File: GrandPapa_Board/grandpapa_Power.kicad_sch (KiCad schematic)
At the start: 31 parts, among them U1 LT1576IS8-5#TRPBF, U11 INA180, U2 TPS61023DRLT, U5 FPF2124

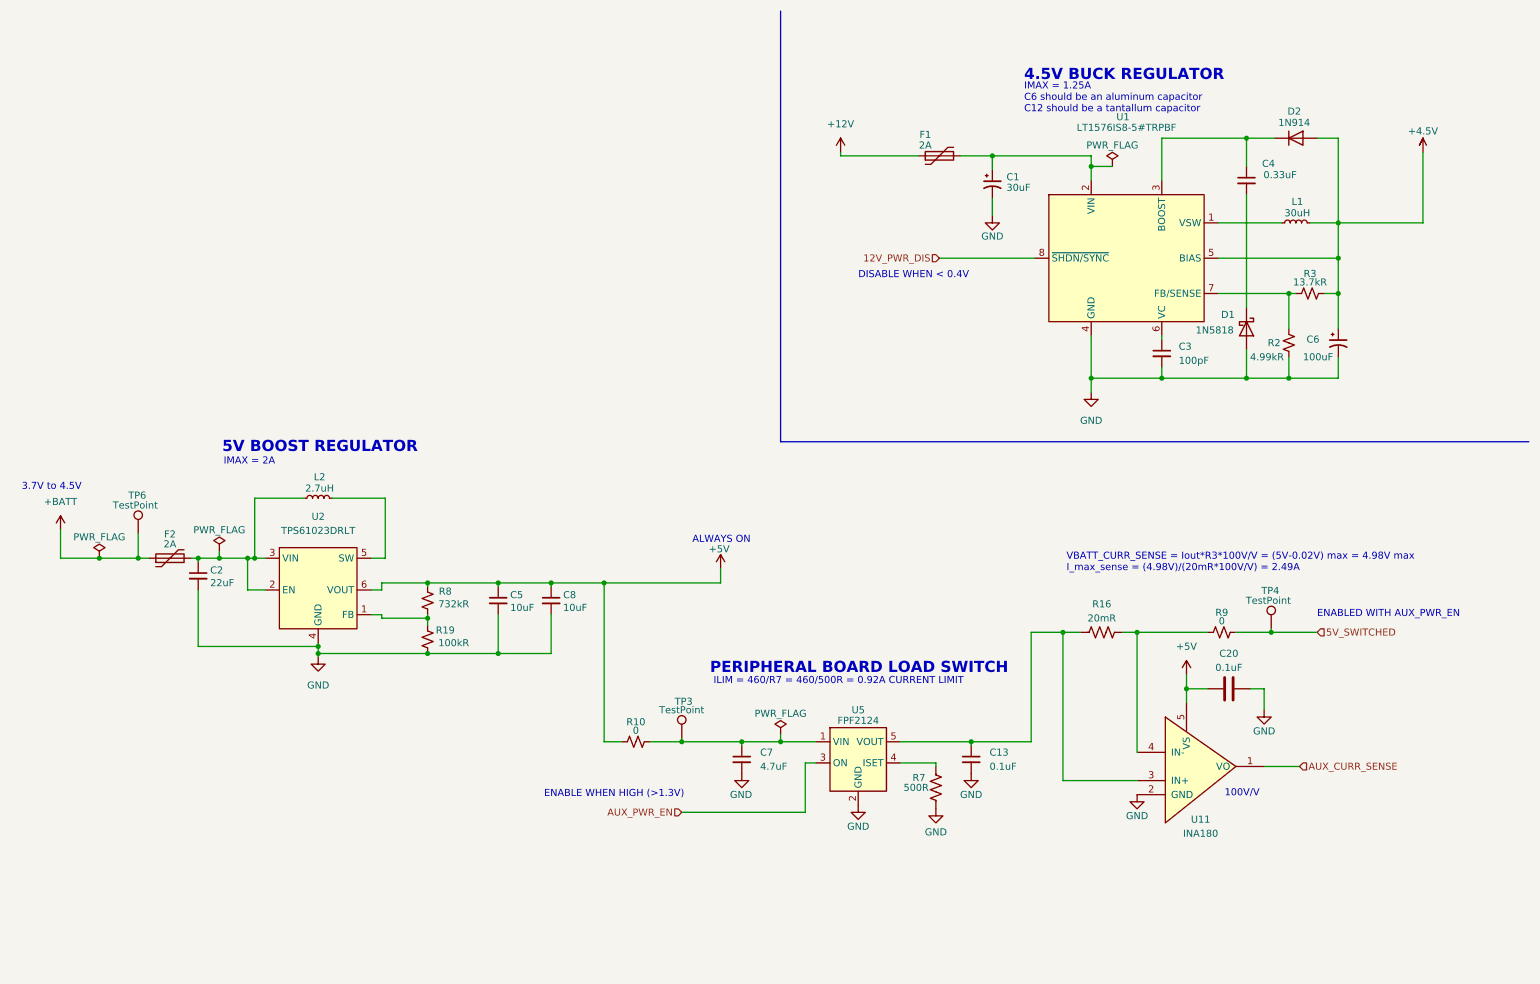
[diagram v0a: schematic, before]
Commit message: Addressed some Jack comments. 3/4/6/7 TBD
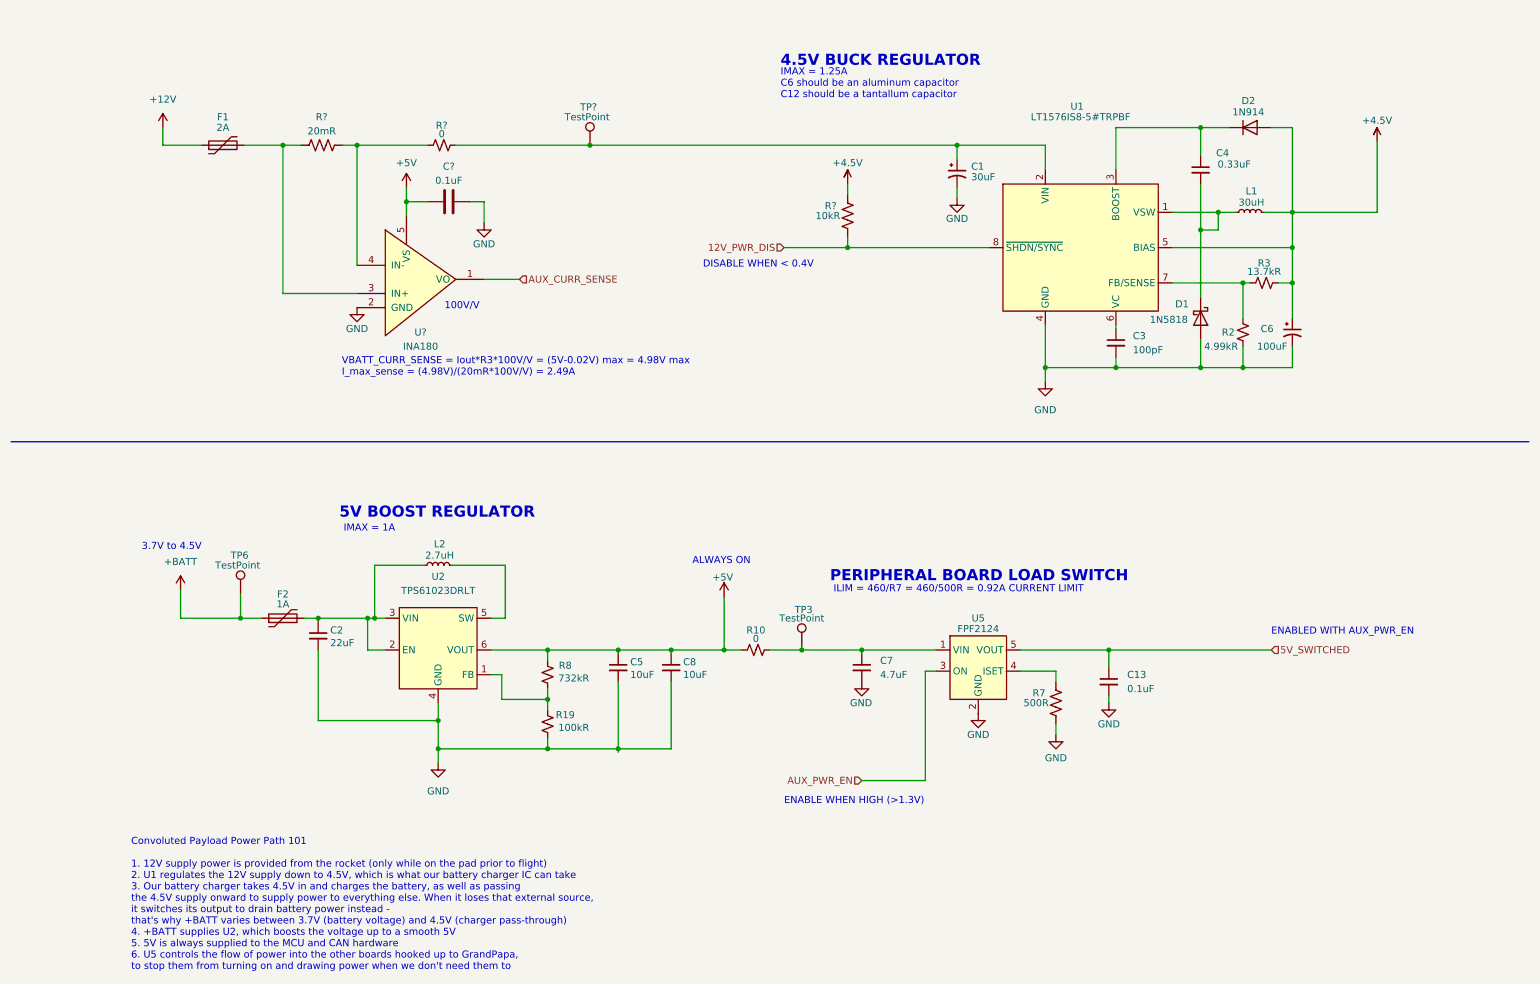
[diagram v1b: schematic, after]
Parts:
- removed C20: 0.1uF, Capacitor_SMD:C_0805_2012Metric_Pad1.18x1.45mm_HandSolder, symbol Device:C
- removed R16: 20mR, Resistor_SMD:R_1206_3216Metric_Pad1.30x1.75mm_HandSolder, symbol Device:R_US
- removed R9: 0, symbol Device:R_Small_US
- removed TP4: TestPoint, Connector_PinHeader_2.54mm:PinHeader_1x01_P2.54mm_Vertical, symbol Connector:TestPoint
- removed U11: INA180, symbol CANHW:INA180
- added C?: 0.1uF, Capacitor_SMD:C_0805_2012Metric_Pad1.18x1.45mm_HandSolder, symbol Device:C
- added R?: 20mR, Resistor_SMD:R_1206_3216Metric_Pad1.30x1.75mm_HandSolder, symbol Device:R_US
- added R?: 0, symbol Device:R_Small_US
- added R?: 10kR, Resistor_SMD:R_1206_3216Metric_Pad1.30x1.75mm_HandSolder, symbol Device:R_US
- added TP?: TestPoint, Connector_PinHeader_2.54mm:PinHeader_1x01_P2.54mm_Vertical, symbol Connector:TestPoint
- added U?: INA180, symbol CANHW:INA180
- F2: value 2A -> 1A
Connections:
- net +4.5V: now also R?.1
- net +5V: now also C?.2, U?.5 (VS)
- net 12V_PWR_DIS: now also R?.2
- net 5V_SWITCHED: now also C13.1, U5.5 (VOUT)
- net AUX_CURR_SENSE: now also U?.1 (VO)
- net GND: now also C?.1, U?.2 (GND)
- net at L1.1, U1.1 (VSW): now also C4.2, D1.1 (K)
- net at C1.1, U1.2 (VIN): now also R?.2, TP?.1; no longer F1.2
- new net: F1.2, R?.2, U?.3 (IN+)
- new net: R?.1, R?.1, U?.4 (IN-)
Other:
- note added: "Convoluted Payload Power Path 101 1. 12V supply power is provided from the rocket (only while on the pad prior to flight) 2. U1 regulates the 12V supply down to 4.5V, which is what our battery charger IC can take 3. Our battery charger takes 4.5V in and charges the battery, as well as passing the 4.5V supply onward to supply power to everything else. When it loses that external source, it switche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"
- note added: "IMAX = 1A"
- note removed: "IMAX = 2A"
- moved on the sheet: C1, C13, C2, C3, C4, C5, C6, C7, C8, D1, D2, F1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
